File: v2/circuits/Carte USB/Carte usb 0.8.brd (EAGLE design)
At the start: 105.4 x 45.4 mm, 15 parts, among them Q1 TIP31C, Q2 TIP31C, Q3 TIP31C, Q4 TIP30, Q5 TIP30, Q6 TIP30, X1 MKS1854-6-0-404, X2 MKS1854-6-0-404, X3 MKS1854-6-0-404

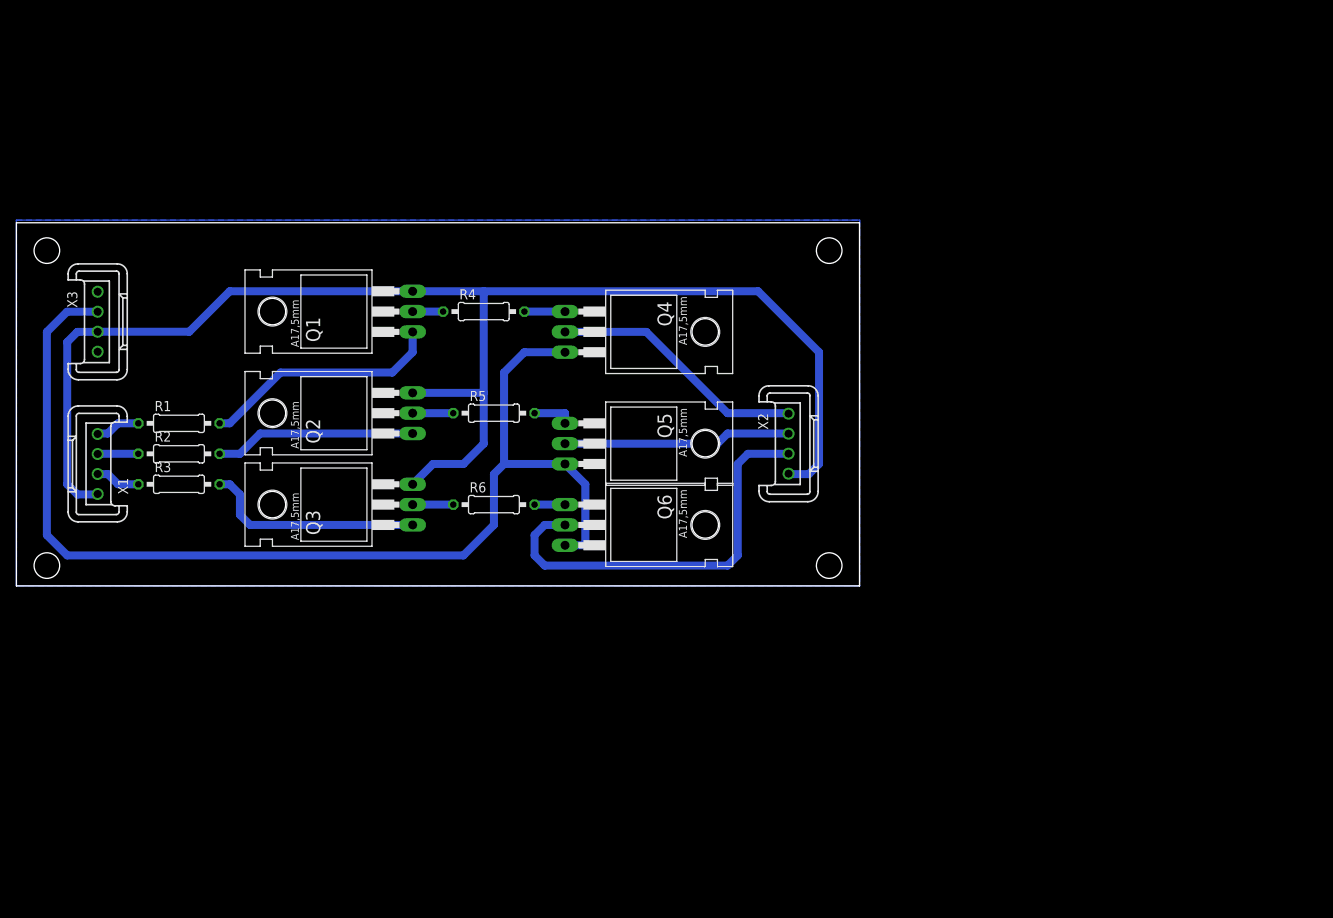
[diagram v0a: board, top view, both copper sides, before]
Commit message: added boards
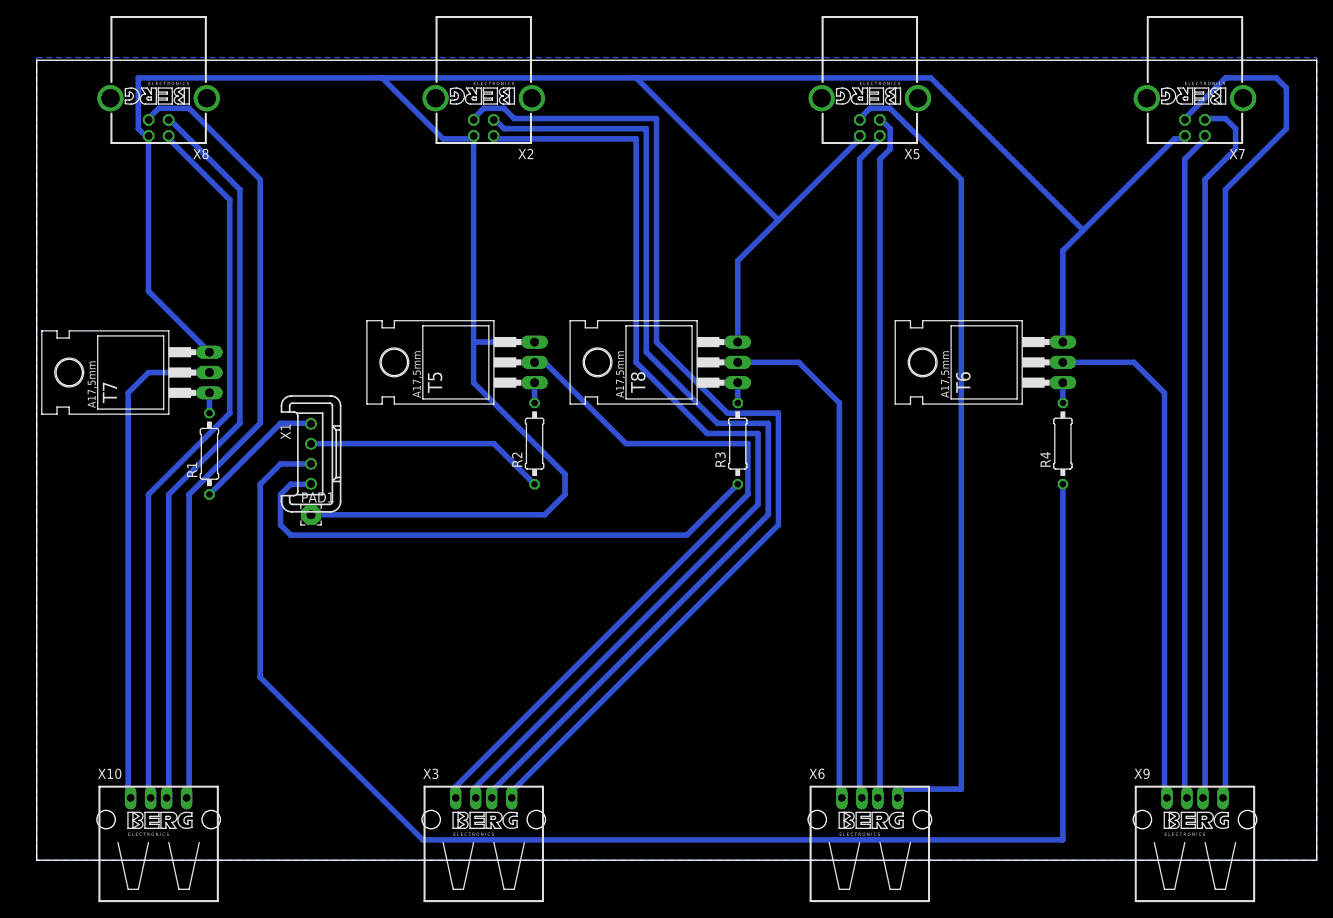
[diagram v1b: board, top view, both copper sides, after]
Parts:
- removed Q1, Q2, Q3: TIP31C, transistor-npn:TO220
- removed Q4, Q5, Q6: TIP30, transistor-pnp:TO220
- removed R5, R6: 1200, resistor:0207/10
- added PAD1: (no value), wirepad:2,54/1,1
- added T5, T6, T7, T8: BDX54, transistor:TO220
- added X10, X6, X9: (no value), con-berg:PN87520
- added X5, X7, X8: PN61729-S, con-berg:PN61729-S
- R1, R2, R3: value 250 -> (none); device resistor:0207/10 -> rcl:0207/10
- R4: value 1200 -> (none); device resistor:0207/10 -> rcl:0207/10
- X2: value MKS1854-6-0-404 -> PN61729-S; device con-stocko:MKS1854-6-0-404 -> con-berg:PN61729-S
- X3: value MKS1854-6-0-404 -> (none); device con-stocko:MKS1854-6-0-404 -> con-berg:PN87520
- moved X3 78.8 mm to (55.9, 5.08), turned to 0 degrees
- moved R4 74.2 mm to (128.3, 52.1), turned to 90 degrees
- moved R3 70.0 mm to (87.6, 52.1), turned to 90 degrees
- moved X2 57.6 mm to (55.9, 95.2), turned to 180 degrees
- moved R2 44.5 mm to (62.2, 52.1), turned to 90 degrees
- moved X1 26.7 mm to (34.3, 50.8), turned to 270 degrees
- moved R1 5.39 mm to (21.6, 50.8), turned to 90 degrees
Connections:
- removed net N$3: Q3.1, R3.2
- removed net N$6: Q3.2, R6.1
- new net N$19: X5.4, X6.4
- new net N$20: T6.2, X9.1
- new net N$21: T7.2, X10.1
- new net N$22: X7.4, X9.4
- new net N$25: T5.2, X3.1
- new net N$29: R1.2, T7.1
- new net N$30: R1.1, X1.1
- new net N$31: R2.1, X1.2
- new net N$32: R4.1, X1.3
- new net N$33: R3.1, X1.4
- net N$1: now also R2.2, T5.1; no longer Q1.1, R1.2
- net N$10: now also X5.2, X6.2; no longer Q1.3, Q2.3, Q3.3, X1.1, X2.4, X3.3
- net N$12: now also X7.2, X9.2; no longer R1.1, X1.4
- net N$13: now also X2.4, X3.4; no longer R2.1, X1.3
- net N$14: now also X7.3, X9.3; no longer R3.1, X1.2
- net N$15: now also PAD1.1, T5.3, T6.3, T7.3, T8.3, X2.1, X5.1, X7.1, X8.1; no longer Q4.3, Q5.3, Q6.3, X3.2
- net N$16: now also X10.2, X8.2; no longer Q4.2, X2.1
- net N$17: now also X10.3, X8.3; no longer Q5.2, X2.2
- net N$18: now also X10.4, X8.4; no longer Q6.2, X2.3
- net N$2: now also R3.2, T8.1; no longer Q2.1, R2.2
- net N$4: now also X2.2, X3.2; no longer Q1.2, R4.1
- net N$5: now also R4.2, T6.1; no longer Q2.2, R5.1
- net N$7: now also X2.3, X3.3; no longer Q4.1, R4.2
- net N$8: now also X5.3, X6.3; no longer Q5.1, R5.2
- net N$9: now also T8.2, X6.1; no longer Q6.1, R6.2
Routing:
- net N$11: track 302.3 -> 0.00 mm
- net N$15: track 140.9 -> 359.0 mm
- net N$32: track 0.00 -> 184.7 mm
- net N$13: track 5.10 -> 132.8 mm
- net N$7: track 5.08 -> 127.7 mm
- net N$4: track 3.81 -> 125.3 mm
- net N$22: track 2.54 -> 107.4 mm
- net N$19: track 2.54 -> 102.0 mm
- net N$10: track 179.3 -> 83.8 mm
- net N$25: track 2.54 -> 90.5 mm
- net N$14: track 5.61 -> 89.7 mm
- net N$8: track 5.08 -> 86.2 mm
- net N$12: track 5.63 -> 83.8 mm
- net N$33: track 0.00 -> 68.5 mm
- net N$17: track 28.5 -> 92.5 mm
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- added copper zone on layer 16, net N$3
- removed copper zone on layer 16, net N$27
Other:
- board size 105.4 x 45.4 mm -> 160 x 100 mm
